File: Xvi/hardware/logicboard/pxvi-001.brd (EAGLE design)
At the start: 91 x 90 mm, 58 parts, among them J0 12V, J1 MKR, J7 DIN5, Q1 60V/32A/35mΩ, Q10 60V/32A/35mΩ, Q11 60V/32A/35mΩ, Q12 60V/32A/35mΩ, Q13 60V/32A/35mΩ, Q14 60V/32A/35mΩ, Q15 60V/32A/35mΩ, Q16 60V/32A/35mΩ, Q2 60V/32A/35mΩ, Q3 60V/32A/35mΩ, Q4 60V/32A/35mΩ, Q5 60V/32A/35mΩ, Q6 60V/32A/35mΩ, Q7 60V/32A/35mΩ, Q8 60V/32A/35mΩ, Q9 60V/32A/35mΩ, U1 DS18B20, X2 ADAFRUIT-PCA9685

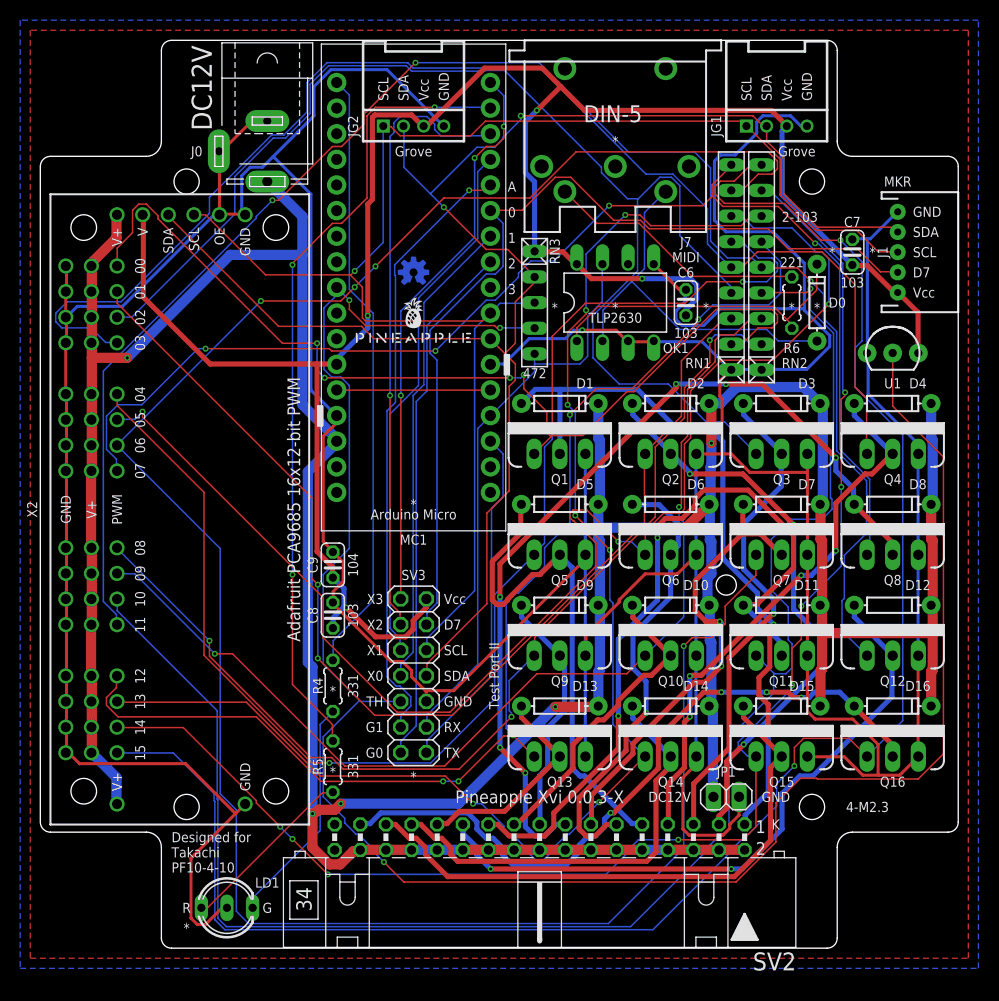
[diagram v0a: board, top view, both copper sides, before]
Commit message: Guide for fan.
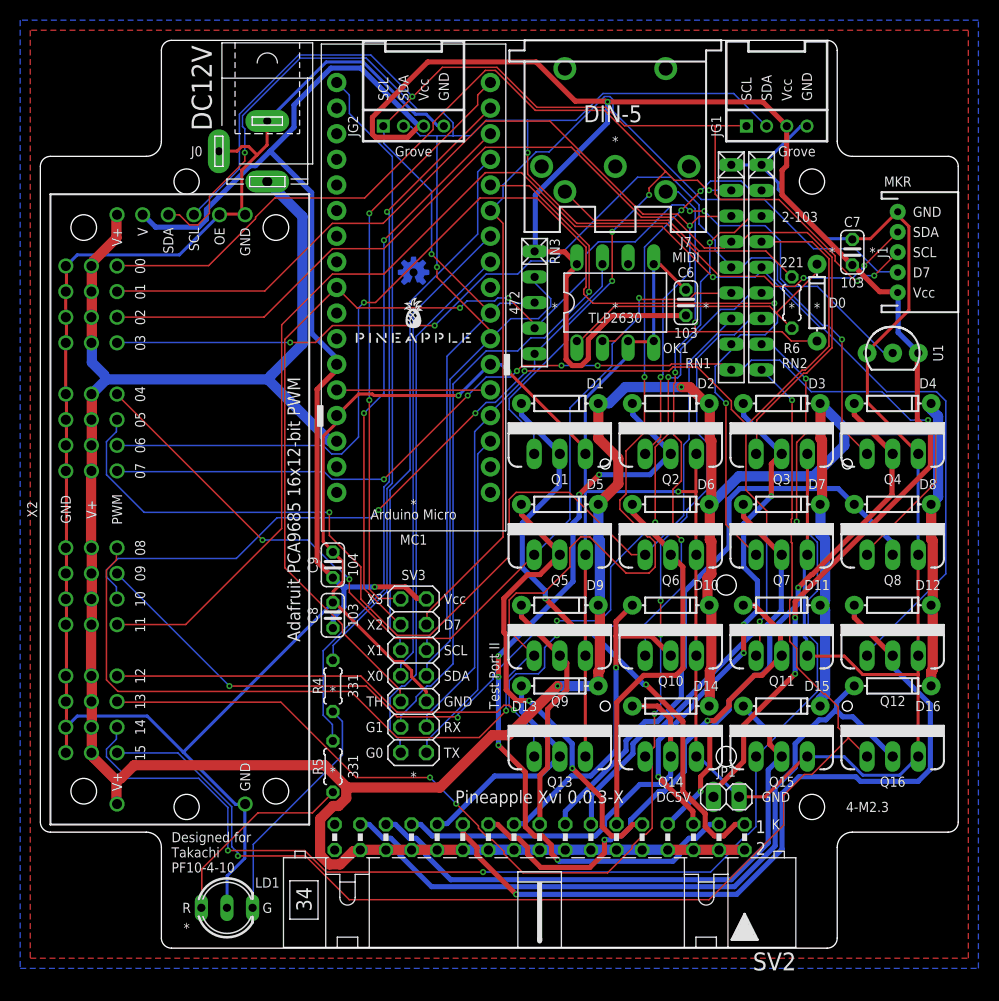
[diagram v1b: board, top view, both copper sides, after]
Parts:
- moved D13 2.00 mm to (51.5, 26.0)
- moved D16 2.00 mm to (84.5, 26.0)
- turned RN1 to 270 degrees
- turned RN2 to 270 degrees
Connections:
- net VCC: now also JP1.1
- net VIN: no longer JP1.1
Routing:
- net PWM06: track 216.4 -> 121.6 mm, vias 4 -> 3
- net GND: track 557.2 -> 468.9 mm, vias 1 -> 3
- net THS: track 197.7 -> 120.5 mm, vias 3 -> 4
- net VCC: track 210.6 -> 284.2 mm
- net PWM15: track 176.3 -> 132.5 mm
- net PWM04: track 134.9 -> 94.9 mm
- net SDA: track 163.1 -> 201.1 mm, vias 2 -> 5
- net PWM08: track 102.7 -> 139.0 mm, vias 3 -> 4
- net PWM10: track 161.6 -> 129.8 mm, vias 1 -> 5
- net PWM05: track 137.0 -> 107.9 mm, vias 3 -> 1
- net PWM03: track 129.7 -> 101.2 mm, vias 0 -> 3
- net LD07: track 87.8 -> 59.8 mm, vias 6 -> 0
- net LD10: track 75.0 -> 50.2 mm
- net VIN: track 399.4 -> 377.4 mm, vias 6 -> 2
- net PWM02: track 127.6 -> 106.5 mm
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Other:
- board text added: "DC5V"
- board text added: "Holes are design guide for 30mm fan"
- board text removed: "0"
- board text removed: "1"
- board text removed: "2"
- board text removed: "3"
- board text removed: "A"
